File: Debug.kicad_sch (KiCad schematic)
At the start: 4 parts, among them J2 Conn_02x10_Odd_Even

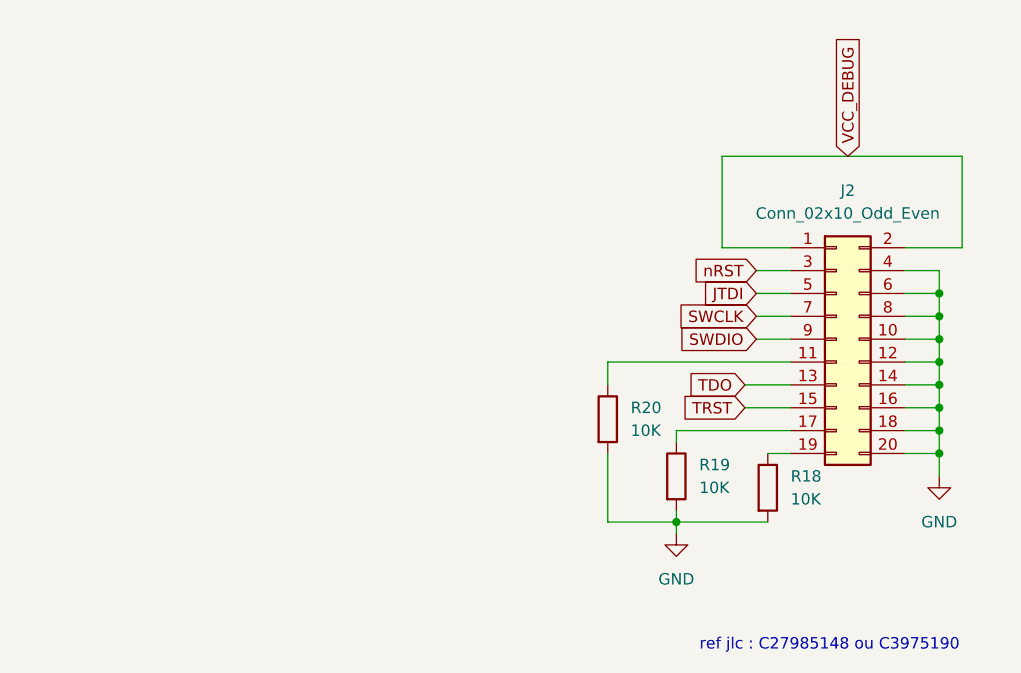
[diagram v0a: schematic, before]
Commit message: Dernieres pour review
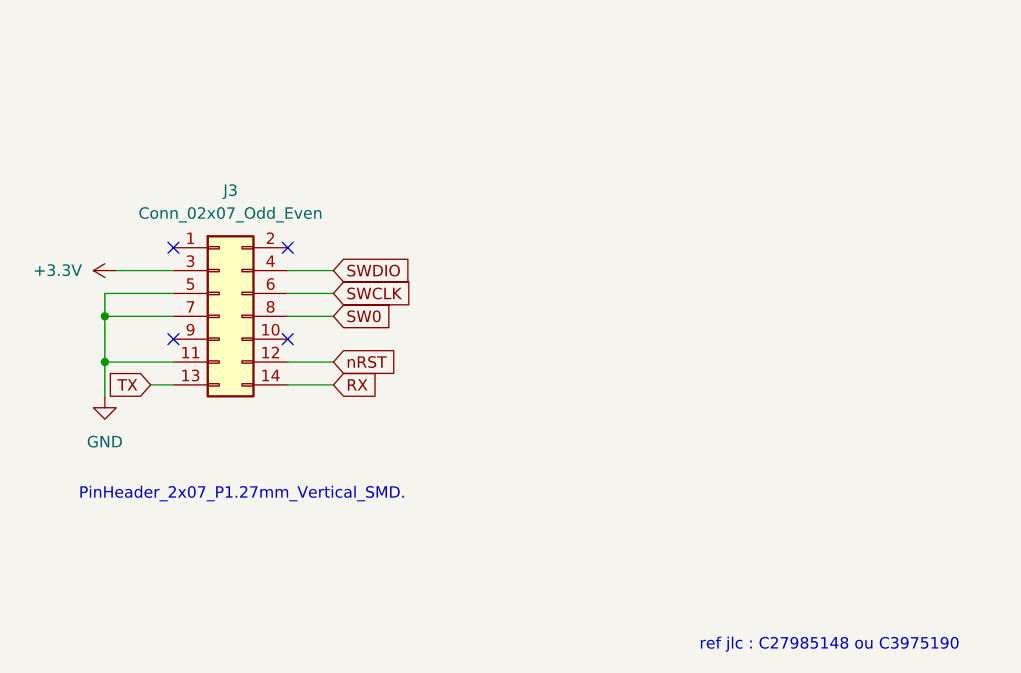
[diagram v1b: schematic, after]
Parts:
- removed J2: Conn_02x10_Odd_Even, symbol Connector_Generic:Conn_02x10_Odd_Even
- removed R18, R19, R20: 10K, symbol Device:R
- added J3: Conn_02x07_Odd_Even, symbol Connector_Generic:Conn_02x07_Odd_Even
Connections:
- net GND: now also J3.11 (Pin_11), J3.5 (Pin_5), J3.7 (Pin_7)
- net SWCLK: now also J3.6 (Pin_6)
- net SWDIO: now also J3.4 (Pin_4)
- net nRST: now also J3.12 (Pin_12)
- new net +3.3V: J3.3 (Pin_3)
- new net RX: J3.14 (Pin_14)
- new net SW0: J3.8 (Pin_8)
- new net TX: J3.13 (Pin_13)
- no-connect marks 0 -> 4
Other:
- note added: "PinHeader_2x07_P1.27mm_Vertical_SMD."
